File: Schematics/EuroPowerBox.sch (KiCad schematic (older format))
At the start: 0 parts

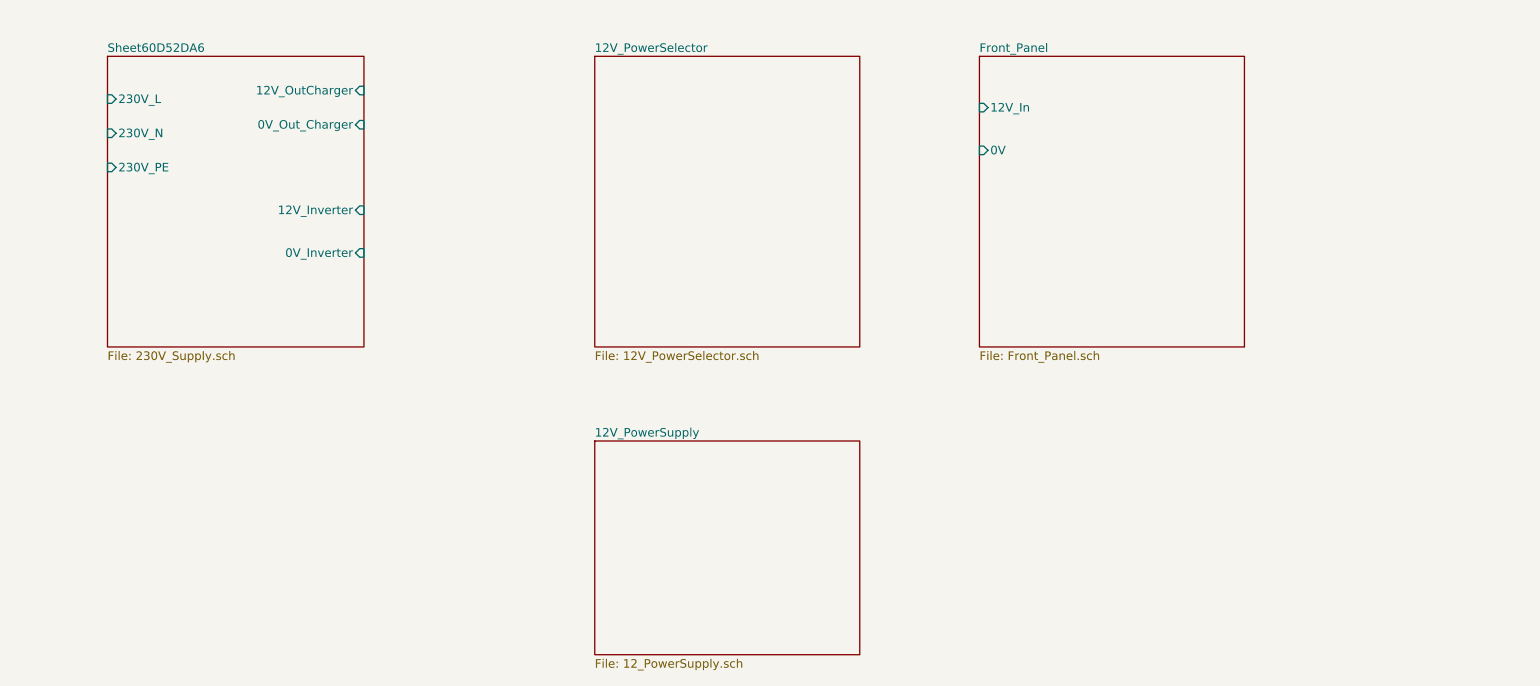
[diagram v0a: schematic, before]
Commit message: Finalize Schematic
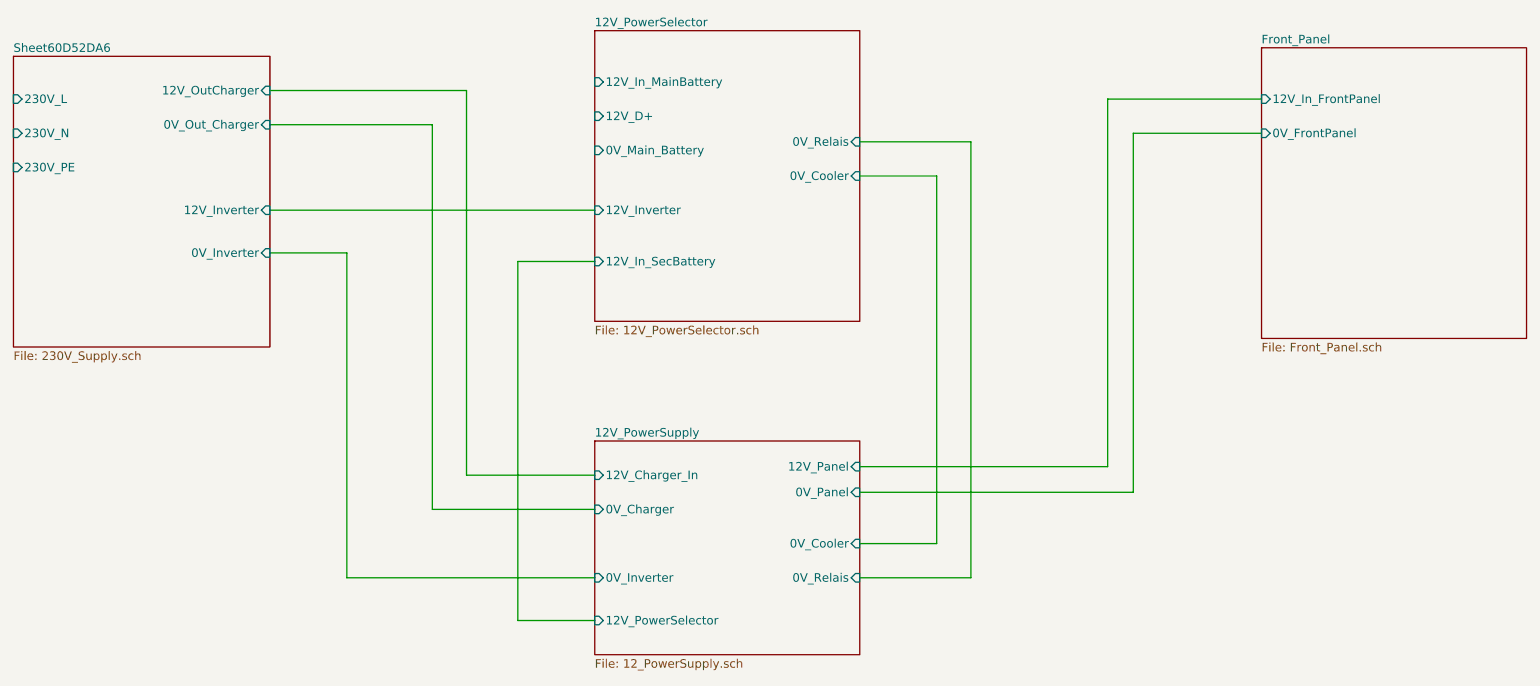
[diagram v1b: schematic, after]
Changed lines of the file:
@@
 $EndDescr
 $Sheet
-S 1600 1850 1500 1700
+S 1050 1850 1500 1700
 U 60D52DA7
 F0 "Sheet60D52DA6" 50
 F1 "230V_Supply.sch" 50
-F2 "230V_L" I L 1600 2100 50
-F3 "230V_N" I L 1600 2300 50
-F4 "230V_PE" I L 1600 2500 50
-F5 "12V_Inverter" I R 3100 2750 50
-F6 "0V_Inverter" I R 3100 3000 50
-F7 "12V_OutCharger" I R 3100 2050 50
-F8 "0V_Out_Charger" I R 3100 2250 50
+F2 "230V_L" I L 1050 2100 50
+F3 "230V_N" I L 1050 2300 50
+F4 "230V_PE" I L 1050 2500 50
+F5 "12V_Inverter" I R 2550 2750 50
+F6 "0V_Inverter" I R 2550 3000 50
+F7 "12V_OutCharger" I R 2550 2050 50
+F8 "0V_Out_Charger" I R 2550 2250 50
 $EndSheet
 $Sheet
-S 4450 1850 1550 1700
+S 4450 1700 1550 1700
 U 60D52DDD
 F0 "12V_PowerSelector" 50
 F1 "12V_PowerSelector.sch" 50
+F2 "12V_In_MainBattery" I L 4450 2000 50
+F3 "12V_In_SecBattery" I L 4450 3050 50
+F4 "0V_Relais" I R 6000 2350 50
+F5 "12V_D+" I L 4450 2200 50
+F6 "0V_Cooler" I R 6000 2550 50
+F7 "0V_Main_Battery" I L 4450 2400 50
+F8 "12V_Inverter" I L 4450 2750 50
 $EndSheet
 $Sheet
-S 6700 1850 1550 1700
+S 8350 1800 1550 1700
 U 60D52E4F
 F0 "Front_Panel" 50
 F1 "Front_Panel.sch" 50
-F2 "12V_In" I L 6700 2150 50
-F3 "0V" I L 6700 2400 50
+F2 "12V_In_FrontPanel" I L 8350 2100 50
+F3 "0V_FrontPanel" I L 8350 2300 50
 $EndSheet
 $Sheet
@@
 F0 "12V_PowerSupply" 50
 F1 "12_PowerSupply.sch" 50
+F2 "0V_Charger" I L 4450 4500 50
+F3 "12V_Panel" I R 6000 4250 50
+F4 "0V_Inverter" I L 4450 4900 50
+F5 "0V_Relais" I R 6000 4900 50
+F6 "0V_Cooler" I R 6000 4700 50
+F7 "12V_Charger_In" I L 4450 4300 50
+F8 "12V_PowerSelector" I L 4450 5150 50
+F9 "0V_Panel" I R 6000 4400 50
 $EndSheet
+Wire Wire Line
+	2550 2050 3700 2050
+Wire Wire Line
+	3700 2050 3700 4300
+Wire Wire Line
+	3700 4300 4450 4300
+Wire Wire Line
+	2550 2250 3500 2250
+Wire Wire Line
+	3500 2250 3500 4500
+Wire Wire Line
+	3500 4500 4450 4500
+Wire Wire Line
+	2550 3000 3000 3000
+Wire Wire Line
+	3000 3000 3000 4900
+Wire Wire Line
+	3000 4900 4450 4900
+Wire Wire Line
+	6000 2350 6650 2350
+Wire Wire Line
+	6650 2350 6650 4900
+Wire Wire Line
+	6650 4900 6000 4900
+Wire Wire Line
+	6000 4700 6450 4700
+Wire Wire Line
+	6450 4700 6450 2550
+Wire Wire Line
+	6450 2550 6000 2550
+Wire Wire Line
+	2550 2750 4450 2750
+Wire Wire Line
+	4450 3050 4000 3050
+Wire Wire Line
+	4000 3050 4000 5150
+Wire Wire Line
+	4000 5150 4450 5150
+Wire Wire Line
+	6000 4250 7450 4250
+Wire Wire Line
+	7450 4250 7450 2100
+Wire Wire Line
+	7450 2100 8350 2100
+Wire Wire Line
+	6000 4400 7600 4400
+Wire Wire Line
+	7600 4400 7600 2300
+Wire Wire Line
+	7600 2300 8350 2300
 $EndSCHEMATC
